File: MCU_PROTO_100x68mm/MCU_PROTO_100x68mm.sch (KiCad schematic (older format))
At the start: 15 parts, among them J1 Screw_Terminal_01x03, J10 Conn_01x01_Male, J2 Screw_Terminal_01x03, J3 Conn_01x20_Female, J4 Conn_01x20_Female, J5 Conn_01x20_Female, J6 Conn_01x20_Female, J7 Conn_01x20_Female, J8 Conn_01x20_Female, J9 Conn_01x01_Male

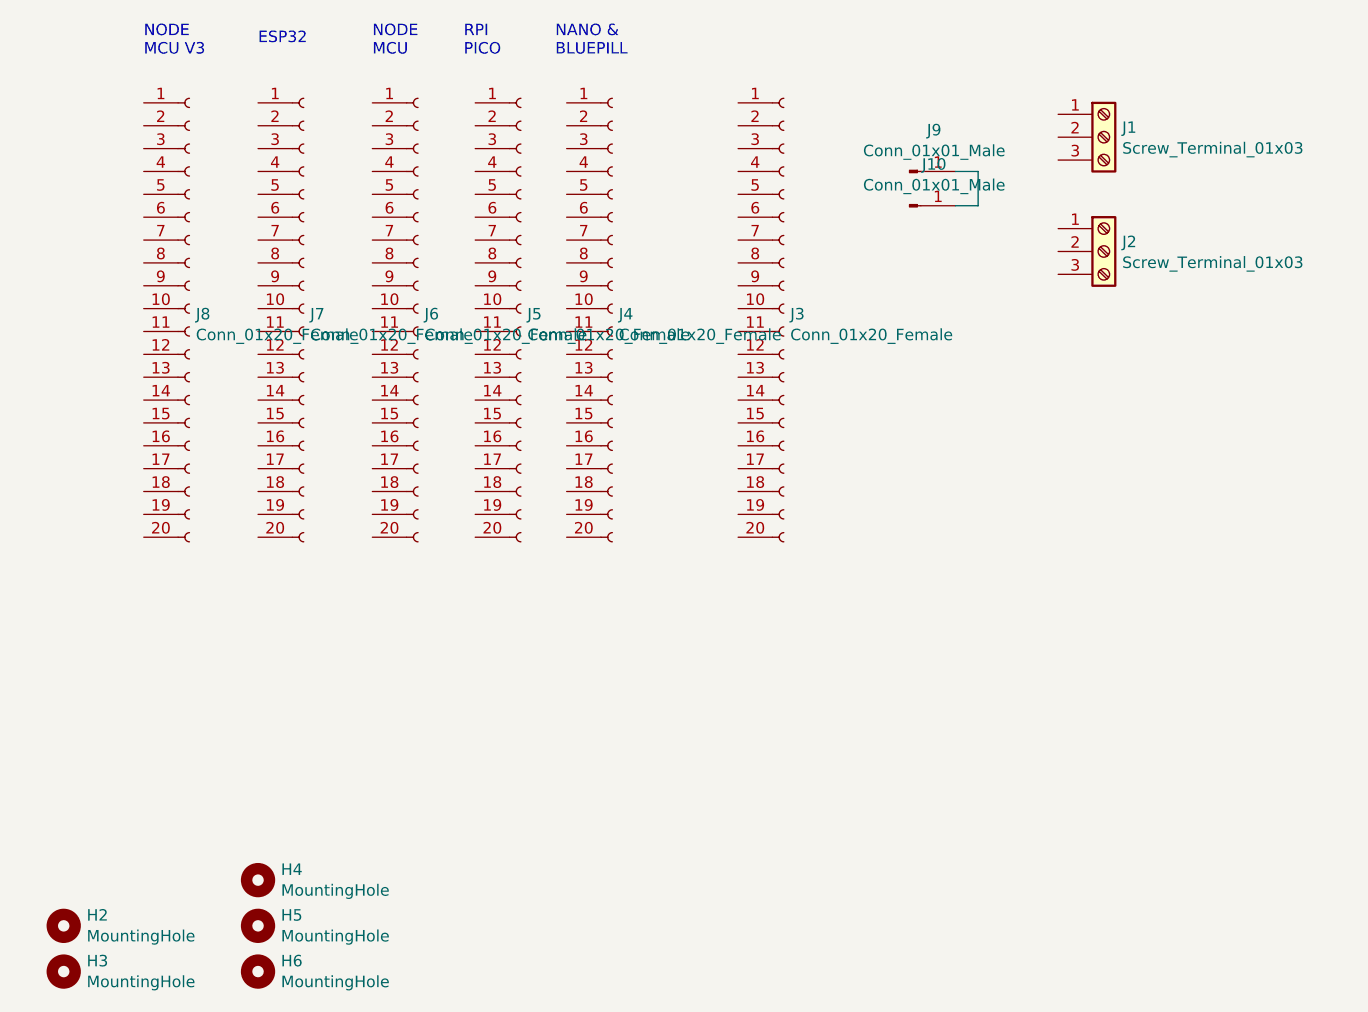
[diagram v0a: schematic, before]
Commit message: all pads placed
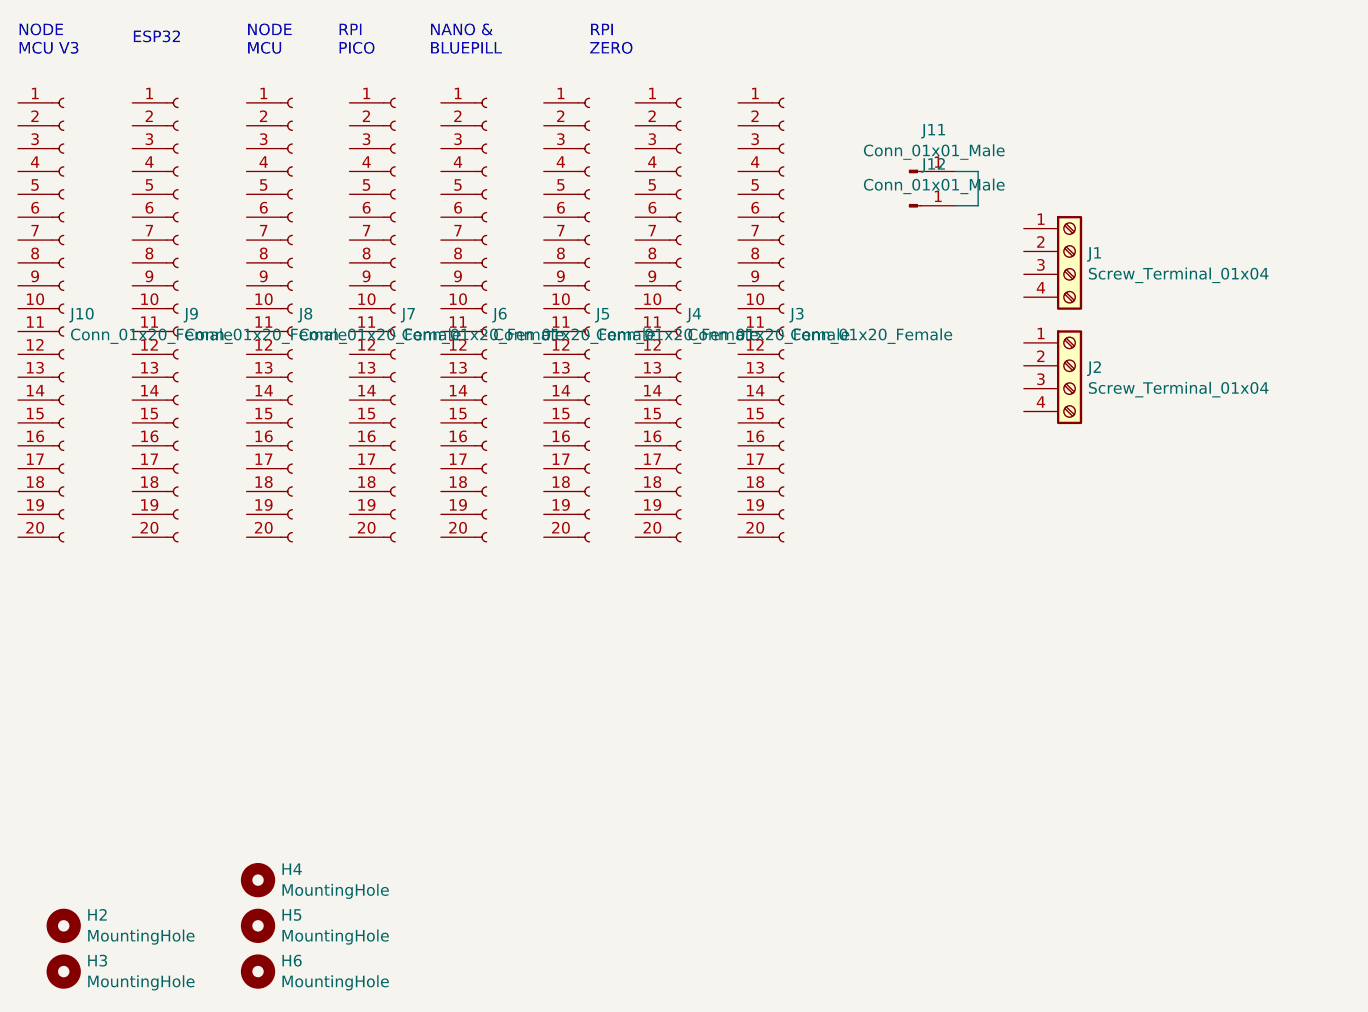
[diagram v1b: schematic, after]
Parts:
- removed J1, J2: Screw_Terminal_01x03, TerminalBlock_4Ucon:TerminalBlock_4Ucon_1x03_P3.50mm_Horizontal, symbol Connector:Screw_Terminal_01x03
- added J1, J2: Screw_Terminal_01x04, TerminalBlock_4Ucon:TerminalBlock_4Ucon_1x04_P3.50mm_Horizontal, symbol Connector:Screw_Terminal_01x04
- added J4, J5: Conn_01x20_Female, Connector_PinSocket_2.54mm:PinSocket_1x20_P2.54mm_Vertical, symbol Connector:Conn_01x20_Female
- renumbered J8 to J10, J9 to J11, J10 to J12, J4 to J6, J5 to J7, J6 to J8, J7 to J9
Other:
- note added: "RPI\nZERO"
- moved on the sheet: J10, J6, J7, J8, J9
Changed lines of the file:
@@
 $EndComp
 $Comp
-L Connector:Screw_Terminal_01x03 J2
-U 1 1 6192413A
-P 8150 2300
-F 0 "J2" H 8230 2342 50  0000 L CNN
-F 1 "Screw_Terminal_01x03" H 8230 2251 50  0000 L CNN
-F 2 "TerminalBlock_4Ucon:TerminalBlock_4Ucon_1x03_P3.50mm_Horizontal" H 8150 2300 50  0001 C CNN
-F 3 "~" H 8150 2300 50  0001 C CNN
-	1    8150 2300
-	1    0    0    -1
-$EndComp
-$Comp
-L Connector:Screw_Terminal_01x03 J1
-U 1 1 6193835B
-P 8150 1800
-F 0 "J1" H 8230 1842 50  0000 L CNN
-F 1 "Screw_Terminal_01x03" H 8230 1751 50  0000 L CNN
-F 2 "TerminalBlock_4Ucon:TerminalBlock_4Ucon_1x03_P3.50mm_Horizontal" H 8150 1800 50  0001 C CNN
-F 3 "~" H 8150 1800 50  0001 C CNN
-	1    8150 1800
-	1    0    0    -1
-$EndComp
-$Comp
-L Connector:Conn_01x01_Male J9
+L Connector:Conn_01x01_Male J11
 U 1 1 6192FB40
 P 7300 1950
-F 0 "J9" H 7408 2131 50  0000 C CNN
+F 0 "J11" H 7408 2131 50  0000 C CNN
 F 1 "Conn_01x01_Male" H 7408 2040 50  0000 C CNN
 F 2 "Connector_Wire:SolderWirePad_1x01_Drill0.8mm" H 7300 1950 50  0001 C CNN
@@
 $EndComp
 $Comp
-L Connector:Conn_01x01_Male J10
+L Connector:Conn_01x01_Male J12
 U 1 1 61938D6F
 P 7300 2100
-F 0 "J10" H 7408 2281 50  0000 C CNN
+F 0 "J12" H 7408 2281 50  0000 C CNN
 F 1 "Conn_01x01_Male" H 7408 2190 50  0000 C CNN
 F 2 "Connector_Wire:SolderWirePad_1x01_Drill0.8mm" H 7300 2100 50  0001 C CNN
@@
 	7600 2100 7500 2100
 $Comp
-L Connector:Conn_01x20_Female J5
+L Connector:Conn_01x20_Female J7
 U 1 1 619361D7
-P 5600 2550
-F 0 "J5" H 5628 2526 50  0000 L CNN
-F 1 "Conn_01x20_Female" H 5628 2435 50  0000 L CNN
-F 2 "Connector_PinSocket_2.54mm:PinSocket_1x20_P2.54mm_Vertical" H 5600 2550 50  0001 C CNN
-F 3 "~" H 5600 2550 50  0001 C CNN
-	1    5600 2550
+P 5050 2550
+F 0 "J7" H 5078 2526 50  0000 L CNN
+F 1 "Conn_01x20_Female" H 5078 2435 50  0000 L CNN
+F 2 "Connector_PinSocket_2.54mm:PinSocket_1x20_P2.54mm_Vertical" H 5050 2550 50  0001 C CNN
+F 3 "~" H 5050 2550 50  0001 C CNN
+	1    5050 2550
 	1    0    0    -1
 $EndComp
@@
 	1    0    0    -1
 $EndComp
-Text Notes 5750 1450 0    50   ~ 0
+Text Notes 5200 1450 0    50   ~ 0
 NANO &\nBLUEPILL
 $Comp
-L Connector:Conn_01x20_Female J4
+L Connector:Conn_01x20_Female J6
 U 1 1 61975404
-P 6000 2550
-F 0 "J4" H 6028 2526 50  0000 L CNN
-F 1 "Conn_01x20_Female" H 6028 2435 50  0000 L CNN
-F 2 "Connector_PinSocket_2.54mm:PinSocket_1x20_P2.54mm_Vertical" H 6000 2550 50  0001 C CNN
-F 3 "~" H 6000 2550 50  0001 C CNN
-	1    6000 2550
+P 5450 2550
+F 0 "J6" H 5478 2526 50  0000 L CNN
+F 1 "Conn_01x20_Female" H 5478 2435 50  0000 L CNN
+F 2 "Connector_PinSocket_2.54mm:PinSocket_1x20_P2.54mm_Vertical" H 5450 2550 50  0001 C CNN
+F 3 "~" H 5450 2550 50  0001 C CNN
+	1    5450 2550
 	1    0    0    -1
 $EndComp
-Text Notes 5350 1450 0    50   ~ 0
+Text Notes 4800 1450 0    50   ~ 0
 RPI\nPICO
 $Comp
-L Connector:Conn_01x20_Female J6
+L Connector:Conn_01x20_Female J8
 U 1 1 6199B975
-P 5150 2550
-F 0 "J6" H 5178 2526 50  0000 L CNN
-F 1 "Conn_01x20_Female" H 5178 2435 50  0000 L CNN
-F 2 "Connector_PinSocket_2.54mm:PinSocket_1x20_P2.54mm_Vertical" H 5150 2550 50  0001 C CNN
-F 3 "~" H 5150 2550 50  0001 C CNN
-	1    5150 2550
+P 4600 2550
+F 0 "J8" H 4628 2526 50  0000 L CNN
+F 1 "Conn_01x20_Female" H 4628 2435 50  0000 L CNN
+F 2 "Connector_PinSocket_2.54mm:PinSocket_1x20_P2.54mm_Vertical" H 4600 2550 50  0001 C CNN
+F 3 "~" H 4600 2550 50  0001 C CNN
+	1    4600 2550
 	1    0    0    -1
 $EndComp
-Text Notes 4950 1450 0    50   ~ 0
+Text Notes 4400 1450 0    50   ~ 0
 NODE\nMCU
 $Comp
-L Connector:Conn_01x20_Female J7
+L Connector:Conn_01x20_Female J9
 U 1 1 619B2BAA
-P 4650 2550
-F 0 "J7" H 4678 2526 50  0000 L CNN
-F 1 "Conn_01x20_Female" H 4678 2435 50  0000 L CNN
-F 2 "Connector_PinSocket_2.54mm:PinSocket_1x20_P2.54mm_Vertical" H 4650 2550 50  0001 C CNN
-F 3 "~" H 4650 2550 50  0001 C CNN
-	1    4650 2550
+P 4100 2550
+F 0 "J9" H 4128 2526 50  0000 L CNN
+F 1 "Conn_01x20_Female" H 4128 2435 50  0000 L CNN
+F 2 "Connector_PinSocket_2.54mm:PinSocket_1x20_P2.54mm_Vertical" H 4100 2550 50  0001 C CNN
+F 3 "~" H 4100 2550 50  0001 C CNN
+	1    4100 2550
 	1    0    0    -1
 $EndComp
-Text Notes 4450 1400 0    50   ~ 0
+Text Notes 3900 1400 0    50   ~ 0
 ESP32
 $Comp
-L Connector:Conn_01x20_Female J8
+L Connector:Conn_01x20_Female J10
 U 1 1 619DA776
-P 4150 2550
-F 0 "J8" H 4178 2526 50  0000 L CNN
-F 1 "Conn_01x20_Female" H 4178 2435 50  0000 L CNN
-F 2 "Connector_PinSocket_2.54mm:PinSocket_1x20_P2.54mm_Vertical" H 4150 2550 50  0001 C CNN
-F 3 "~" H 4150 2550 50  0001 C CNN
-	1    4150 2550
+P 3600 2550
+F 0 "J10" H 3628 2526 50  0000 L CNN
+F 1 "Conn_01x20_Female" H 3628 2435 50  0000 L CNN
+F 2 "Connector_PinSocket_2.54mm:PinSocket_1x20_P2.54mm_Vertical" H 3600 2550 50  0001 C CNN
+F 3 "~" H 3600 2550 50  0001 C CNN
+	1    3600 2550
 	1    0    0    -1
 $EndComp
-Text Notes 3950 1450 0    50   ~ 0
+Text Notes 3400 1450 0    50   ~ 0
 NODE\nMCU V3
 $Comp
@@
 	1    0    0    -1
 $EndComp
+$Comp
+L Connector:Screw_Terminal_01x04 J1
+U 1 1 6205AFF1
+P 8000 2300
+F 0 "J1" H 8080 2292 50  0000 L CNN
+F 1 "Screw_Terminal_01x04" H 8080 2201 50  0000 L CNN
+F 2 "TerminalBlock_4Ucon:TerminalBlock_4Ucon_1x04_P3.50mm_Horizontal" H 8000 2300 50  0001 C CNN
+F 3 "~" H 8000 2300 50  0001 C CNN
+	1    8000 2300
+	1    0    0    -1
+$EndComp
+$Comp
+L Connector:Screw_Terminal_01x04 J2
+U 1 1 620623BF
+P 8000 2800
+F 0 "J2" H 8080 2792 50  0000 L CNN
+F 1 "Screw_Terminal_01x04" H 8080 2701 50  0000 L CNN
+F 2 "TerminalBlock_4Ucon:TerminalBlock_4Ucon_1x04_P3.50mm_Horizontal" H 8000 2800 50  0001 C CNN
+F 3 "~" H 8000 2800 50  0001 C CNN
+	1    8000 2800
+	1    0    0    -1
+$EndComp
+$Comp
+L Connector:Conn_01x20_Female J4
+U 1 1 620E2449
+P 6300 2550
+F 0 "J4" H 6328 2526 50  0000 L CNN
+F 1 "Conn_01x20_Female" H 6328 2435 50  0000 L CNN
+F 2 "Connector_PinSocket_2.54mm:PinSocket_1x20_P2.54mm_Vertical" H 6300 2550 50  0001 C CNN
+F 3 "~" H 6300 2550 50  0001 C CNN
+	1    6300 2550
+	1    0    0    -1
+$EndComp
+$Comp
+L Connector:Conn_01x20_Female J5
+U 1 1 620EBCC7
+P 5900 2550
+F 0 "J5" H 5928 2526 50  0000 L CNN
+F 1 "Conn_01x20_Female" H 5928 2435 50  0000 L CNN
+F 2 "Connector_PinSocket_2.54mm:PinSocket_1x20_P2.54mm_Vertical" H 5900 2550 50  0001 C CNN
+F 3 "~" H 5900 2550 50  0001 C CNN
+	1    5900 2550
+	1    0    0    -1
+$EndComp
+Text Notes 5900 1450 0    50   ~ 0
+RPI\nZERO
 $EndSCHEMATC
